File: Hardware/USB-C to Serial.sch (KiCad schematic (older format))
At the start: 23 parts, among them IC1 ZT213LEEA, IC2 FT231XS-R, J1 5747844-4, P1 USB_C_Plug_USB2.0

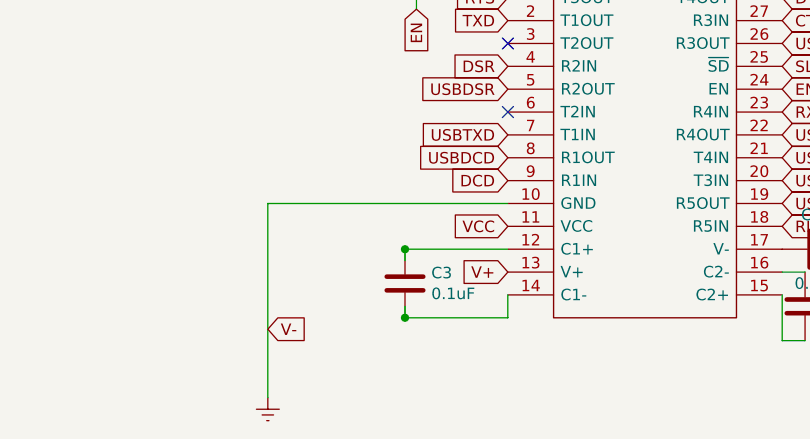
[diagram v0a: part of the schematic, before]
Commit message: Updated files
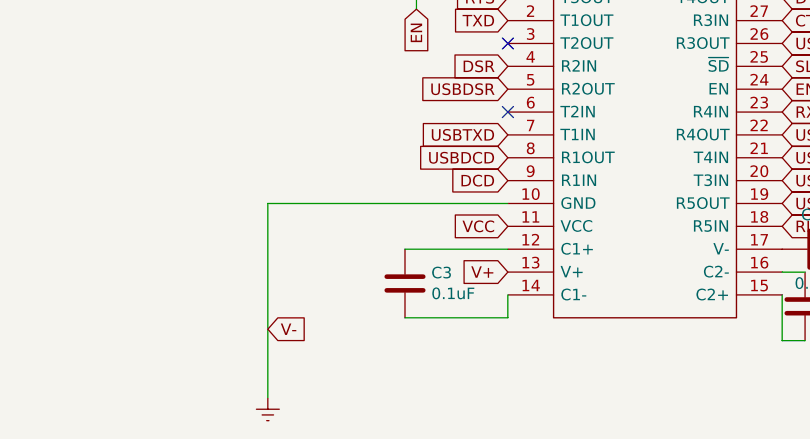
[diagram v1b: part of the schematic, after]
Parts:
- P1: footprint SnapEDA Library:GCT_USB4155-03-C_REVA -> Expansion_Card:USB_C_Plug_Molex_105444
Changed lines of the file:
@@
 F 0 "P1" H 2057 2817 50  0000 C CNN
 F 1 "USB_C_Plug_USB2.0" H 2057 2726 50  0000 C CNN
-F 2 "SnapEDA Library:GCT_USB4155-03-C_REVA" H 2100 1950 50  0001 C CNN
+F 2 "Expansion_Card:USB_C_Plug_Molex_105444" H 2100 1950 50  0001 C CNN
 F 3 "https://www.usb.org/sites/default/files/documents/usb_type-c.zip" H 2100 1950 50  0001 C CNN
 	1    1950 1950
@@
 $EndComp
 Wire Wire Line
-	3500 6450 3500 6500
-Wire Wire Line
-	3500 6250 3500 6200
-Wire Wire Line
 	2900 6000 3950 6000
-Connection ~ 3500 6200
-Connection ~ 3500 6500
 Wire Wire Line
 	3950 6400 3950 6500
